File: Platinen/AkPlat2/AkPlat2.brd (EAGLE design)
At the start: 63.5 x 47.6 mm, 26 parts, among them M1 22-23-2021, M2 22-23-2021, M3 22-23-2021, M4 22-23-2021, X2 332-02, X3 332-02

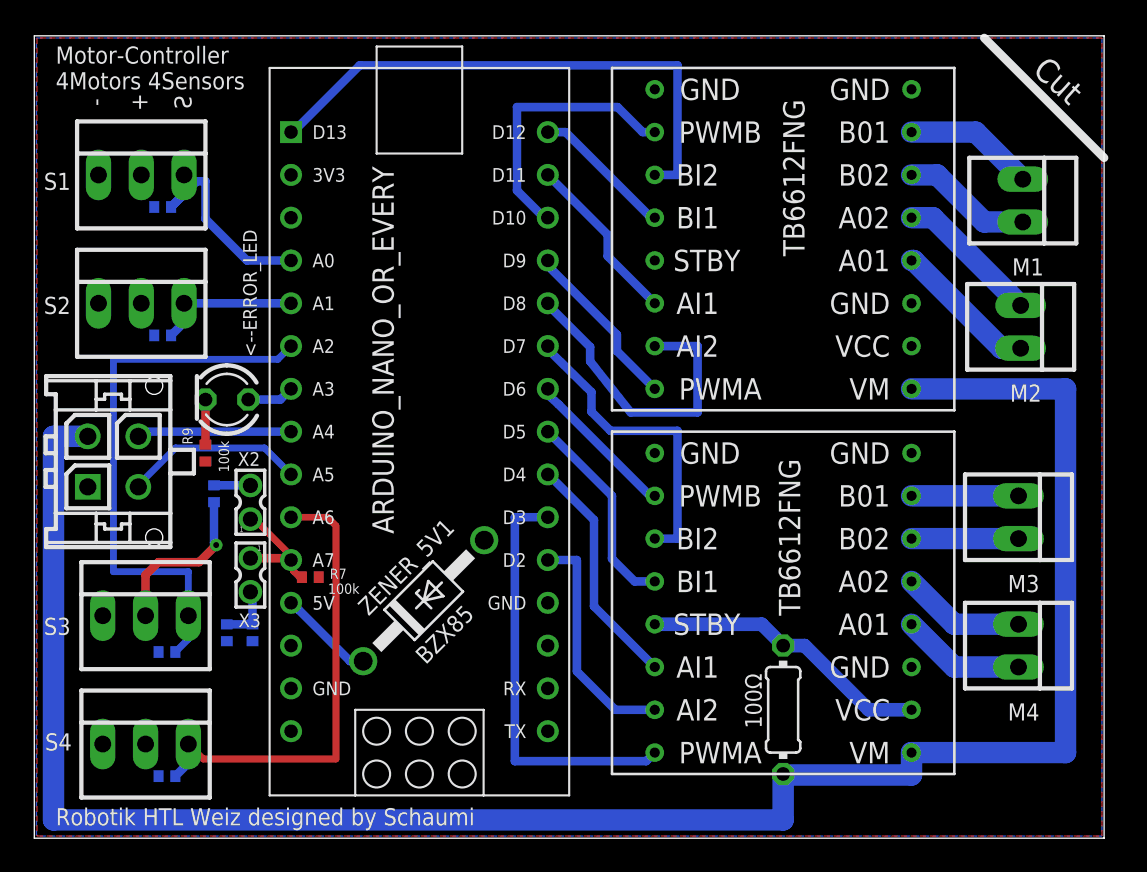
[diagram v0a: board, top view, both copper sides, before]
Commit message: reverted changes
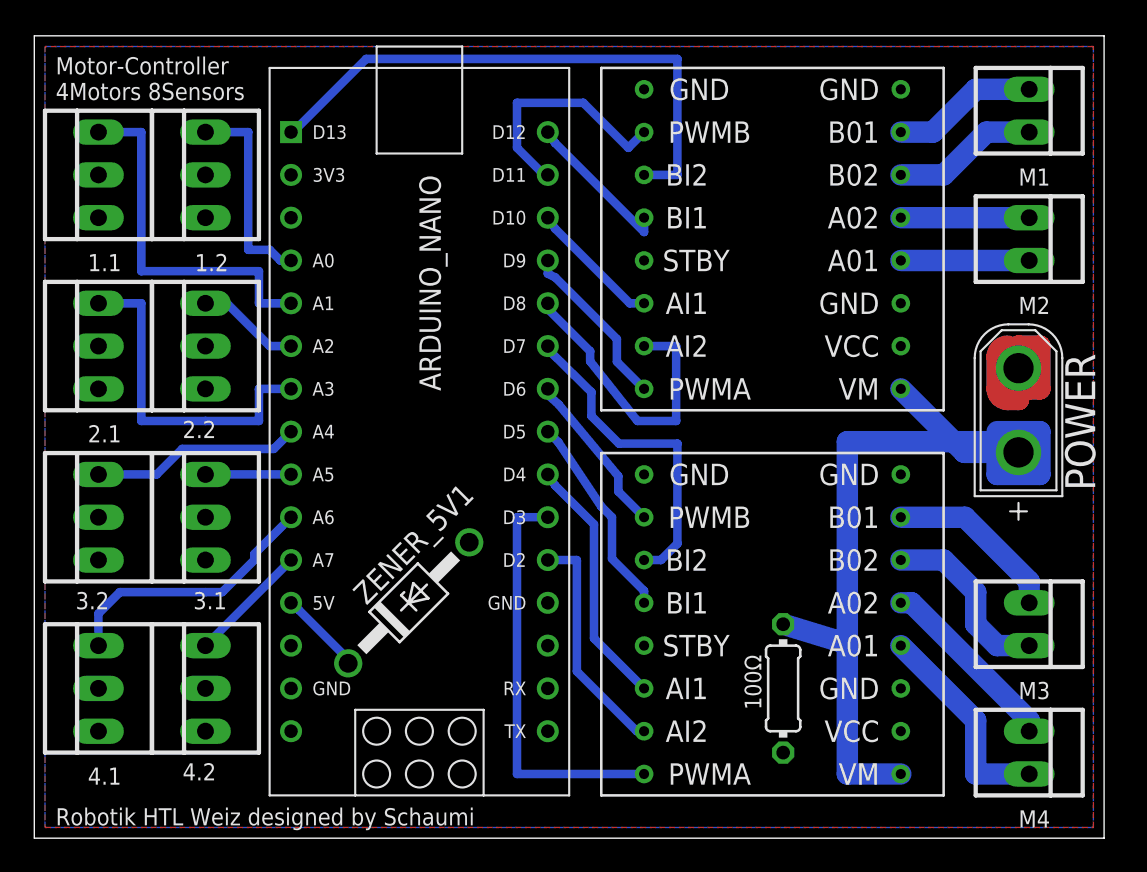
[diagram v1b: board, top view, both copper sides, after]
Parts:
- removed <--ERROR_LED: (no value), led:LED3MM
- removed R1, R2, R3, R4, R5, R6, R7, R8, R9: 100k, rcl:R0402
- removed S1, S2, S3, S4: 22-23-2031, con-molex:22-23-2031
- removed X1: (no value), con-molex-micro-fit-3_0:43045-0412
- removed X2, X3: 332-02, con-garry:332-02
- added 1.1, 1.2, 2.1, 2.2, 3.1, 3.2, 4.1, 4.2: 22-23-2031, con-molex:22-23-2031
- added POWER: XT30UPB-M, amass:XT30UPB-M
- moved M3 6.38 mm to (59.1, 12.7)
- moved M4 6.38 mm to (59.1, 5.08)
- moved M1 5.35 mm to (59.1, 43.2)
- moved M2 5.23 mm to (59.1, 35.6)
- moved U$2 1.42 mm to (54.0, 22.9)
- moved 100Ω 1.27 mm to (44.5, 8.89), turned to 90 degrees
- moved ZENER_5V1 0.90 mm to (22.2, 14.0)
- moved U$1 0.63 mm to (54.0, 45.7)
- renumbered ARDUINO_NANO_OR_EVERY to ARDUINO_NANO
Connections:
- removed net N$1: ARDUINO_NANO.8, X1.P$4
- removed net N$15: R6.1, X2.2
- removed net N$2: ARDUINO_NANO.9, X1.P$3
- removed net N$24: R5.2, R8.2, X3.2
- removed net N$25: <--ERROR_LED.A, ARDUINO_NANO.7
- removed net N$8: ARDUINO_NANO.11, R7.1, X2.1, X3.1
- new net N$27: 4.1.3, ARDUINO_NANO.10
- new net N$30: 3.1.3, ARDUINO_NANO.9
- new net N$31: 3.2.3, ARDUINO_NANO.8
- net 5V: now also 1.1.2, 1.2.2, 2.1.2, 2.2.2, 3.1.2, 3.2.2, 4.1.2, 4.2.2; no longer R1.1, R2.1, R3.1, R4.1, R5.1, R6.2, R8.1, S1.2, S2.2, S3.2, S4.2
- net GND: now also 1.1.1, 1.2.1, 2.1.1, 2.2.1, 3.1.1, 3.2.1, 4.1.1, 4.2.1, POWER.-; no longer R7.2, R9.1, S1.1, S2.1, S3.1, S4.1, X1.P$1
- net N$26: now also 4.2.3, ARDUINO_NANO.11; no longer <--ERROR_LED.K, R9.2
- net N$32: now also 2.1.3, ARDUINO_NANO.7; no longer ARDUINO_NANO.10, R4.2, S4.3
- net N$33: now also 2.2.3; no longer R3.2, S3.3
- net N$34: now also 1.1.3; no longer R2.2, S2.3
- net N$35: now also 1.2.3; no longer R1.2, S1.3
- net N$6: now also ARDUINO_NANO.29; no longer ARDUINO_NANO.28
- net N$7: now also ARDUINO_NANO.28; no longer ARDUINO_NANO.29
- net VM: now also POWER.+; no longer X1.P$2
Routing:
- net VM: track 119.7 -> 54.8 mm
- net 5V: track 33.0 -> 5.01 mm, vias 1 -> 0
- net N$33: track 33.0 -> 6.13 mm
- net N$27: track 0.00 -> 15.9 mm
- net N$34: track 8.57 -> 21.6 mm
- net N$31: track 0.00 -> 12.5 mm
- net GND: track 0.00 -> 11.0 mm
- net N$2: track 10.7 -> 0.00 mm
- net N$1: track 9.18 -> 0.00 mm
- net N$32: track 28.1 -> 20.3 mm
- net N$8: track 7.58 -> 0.00 mm
- net N$23: track 7.40 -> 12.6 mm
- net N$30: track 0.00 -> 5.08 mm
- net N$26: track 2.68 -> 7.18 mm
- net N$21: track 6.35 -> 10.8 mm
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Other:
- board text added: "+"
- board text added: "Motor-Controller 4Motors 8Sensors"
- board text removed: "Cut"
- board text removed: "Motor-Controller 4Motors 4Sensors"
- board text removed: "TB6612FNG"
